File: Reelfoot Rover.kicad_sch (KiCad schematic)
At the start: 2 parts, among them J1 GPIO, U1 7432

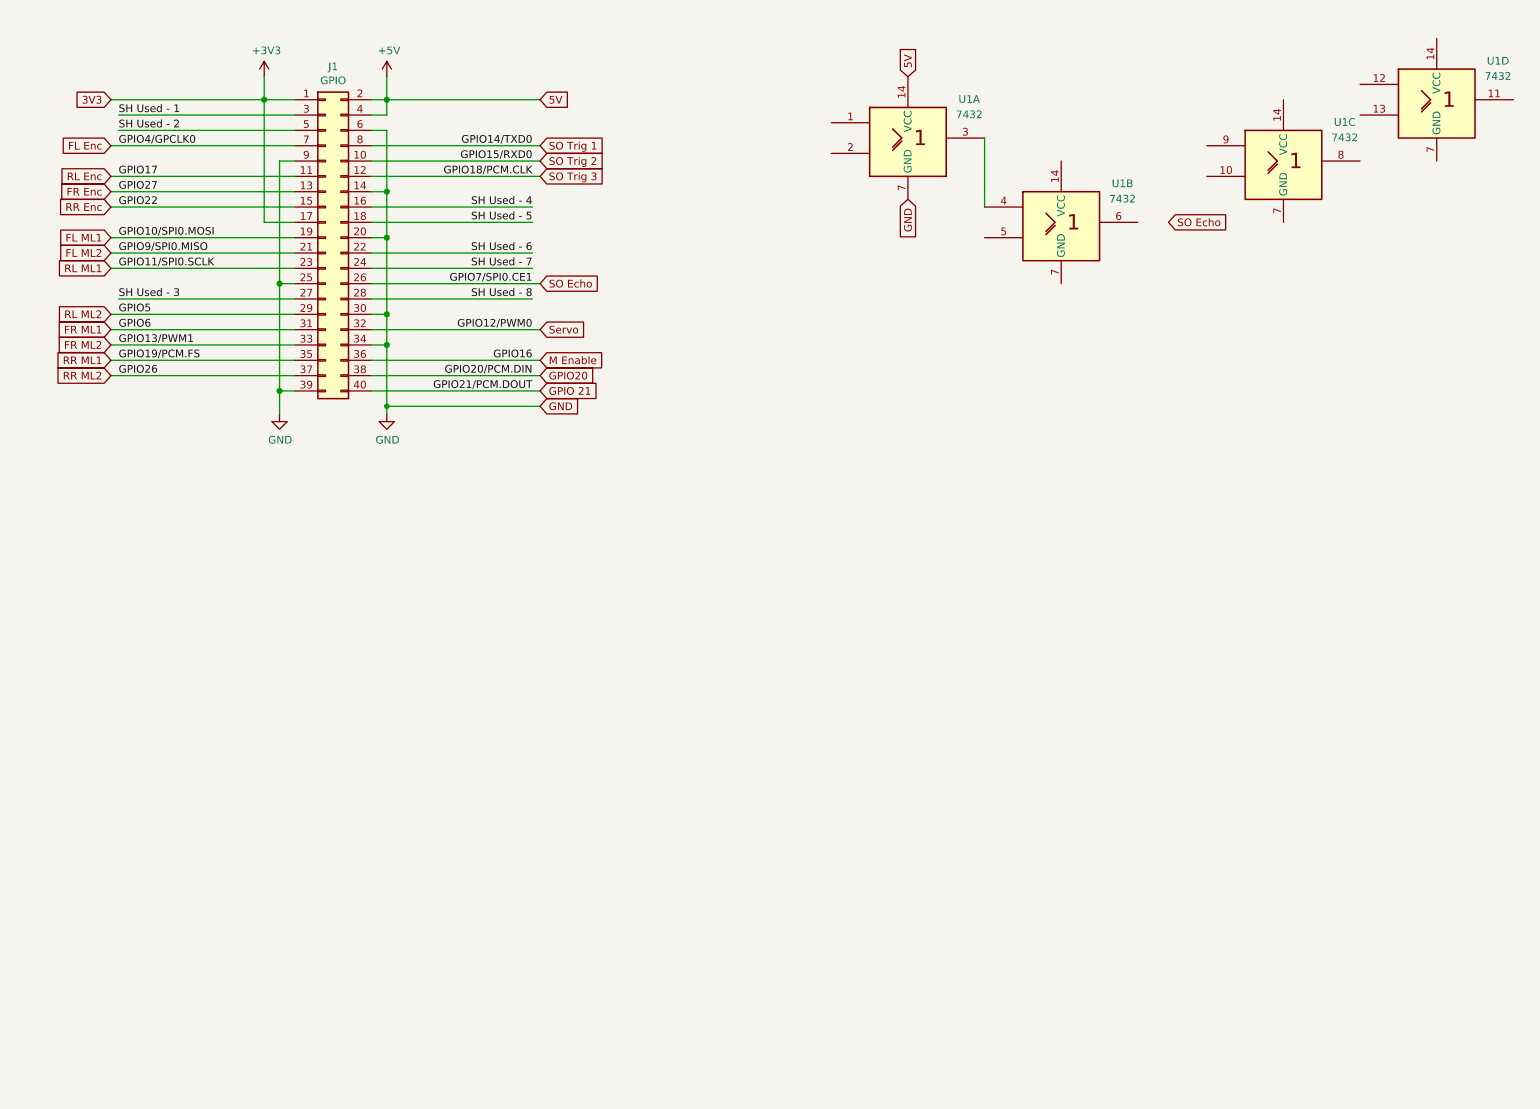
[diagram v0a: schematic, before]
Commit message: first complete draft
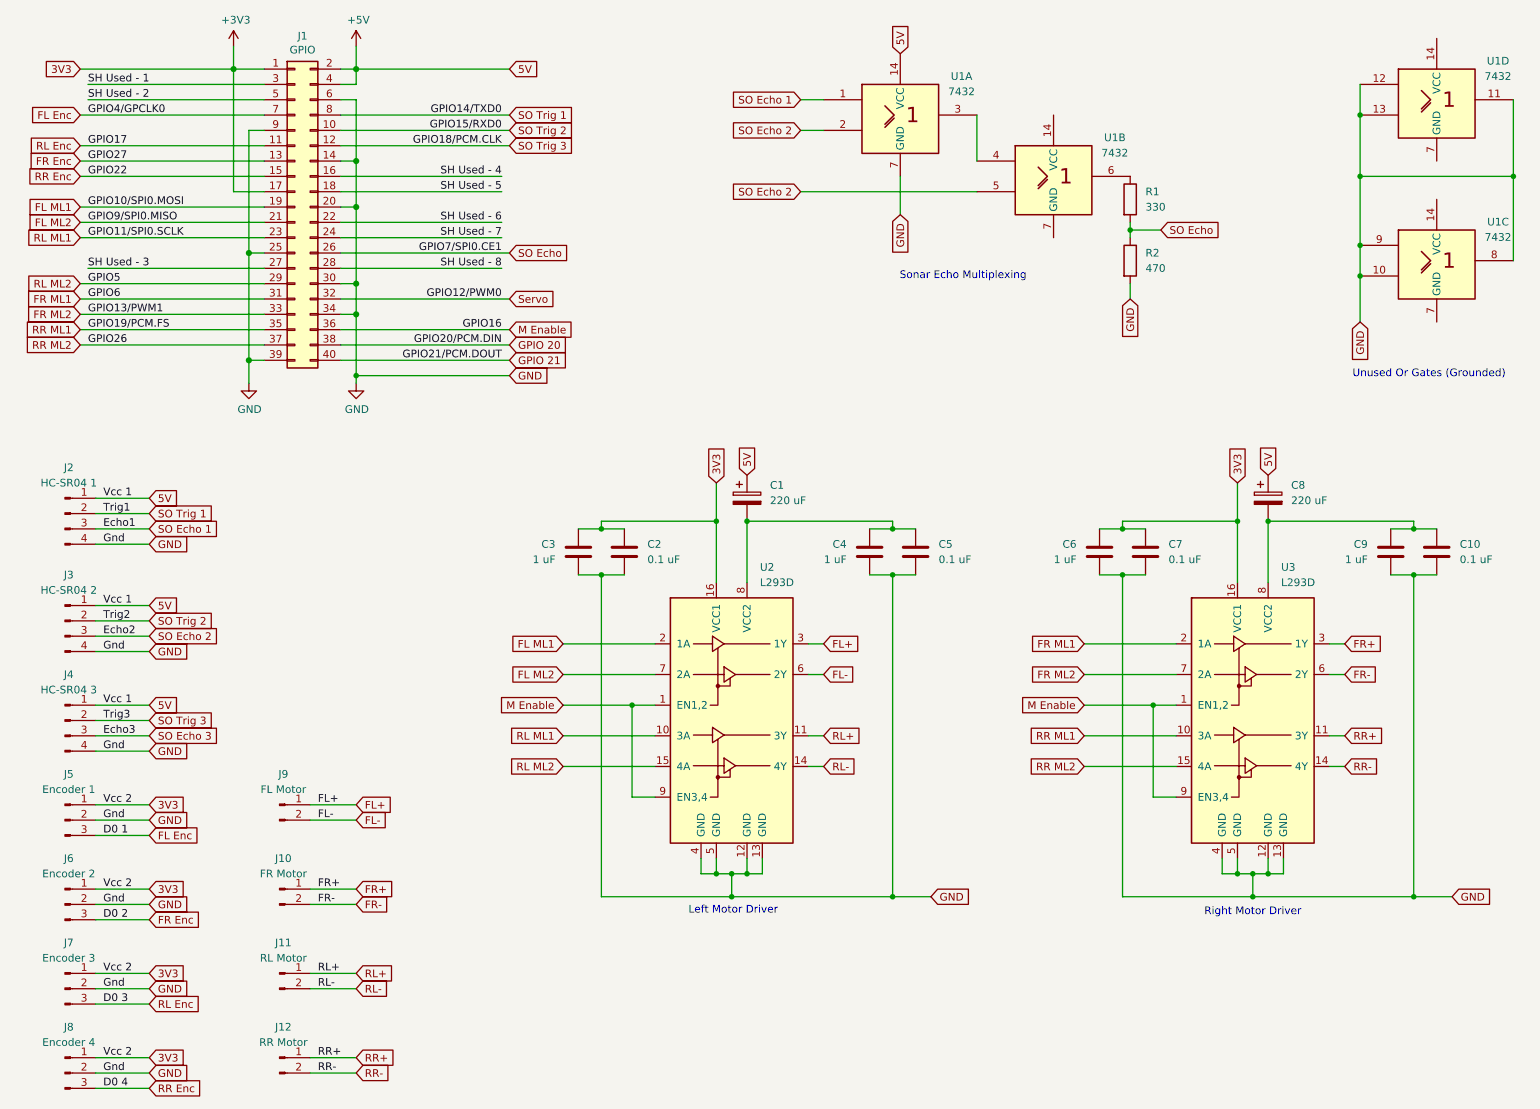
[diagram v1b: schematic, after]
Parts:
- added C1, C8: 220 uF, symbol Device:C_Polarized
- added C10, C2, C5, C7: 0.1 uF, symbol Device:C
- added C3, C4, C6, C9: 1 uF, symbol Device:C
- added J10: FR Motor, symbol Connector:Conn_01x02_Pin
- added J11: RL Motor, symbol Connector:Conn_01x02_Pin
- added J12: RR Motor, symbol Connector:Conn_01x02_Pin
- added J2: HC-SR04 1, symbol Connector:Conn_01x04_Pin
- added J3: HC-SR04 2, symbol Connector:Conn_01x04_Pin
- added J4: HC-SR04 3, symbol Connector:Conn_01x04_Pin
- added J5: Encoder 1, symbol Connector:Conn_01x03_Pin
- added J6: Encoder 2, symbol Connector:Conn_01x03_Pin
- added J7: Encoder 3, symbol Connector:Conn_01x03_Pin
- added J8: Encoder 4, symbol Connector:Conn_01x03_Pin
- added J9: FL Motor, symbol Connector:Conn_01x02_Pin
- added R1: 330, symbol Device:R
- added R2: 470, symbol Device:R
- added U2, U3: L293D, Package_DIP:DIP-16_W7.62mm, symbol Driver_Motor:L293D
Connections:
- net +3V3: now also C2.1, C3.1, C6.1, C7.1, J5.1 (Pin_1), J6.1 (Pin_1), J7.1 (Pin_1), J8.1 (Pin_1), U2.16 (VCC1), U3.16 (VCC1)
- net +5V: now also C1.1, C8.1, J2.1 (Pin_1), J3.1 (Pin_1), J4.1 (Pin_1)
- net FL Enc: now also J5.3 (Pin_3)
- net FL ML1: now also U2.2 (1A)
- net FL ML2: now also U2.7 (2A)
- net FR Enc: now also J6.3 (Pin_3)
- net FR ML1: now also U3.2 (1A)
- net FR ML2: now also U3.7 (2A)
- net GND: now also U1.10, U1.11, U1.12, U1.13, U1.8, U1.9, C10.2, C2.2, C3.2, C4.2, C5.2, C6.2, C7.2, C9.2, J2.4 (Pin_4), J3.4 (Pin_4), J4.4 (Pin_4), J5.2 (Pin_2), J6.2 (Pin_2), J7.2 (Pin_2), J8.2 (Pin_2), R2.2, U2.12 (GND), U2.13 (GND), U2.4 (GND), U2.5 (GND), U3.12 (GND), U3.13 (GND), U3.4 (GND), U3.5 (GND)
- net M Enable: now also U2.1 (EN1,2), U2.9 (EN3,4), U3.1 (EN1,2), U3.9 (EN3,4)
- net RL Enc: now also J7.3 (Pin_3)
- net RL ML1: now also U2.10 (3A)
- net RL ML2: now also U2.15 (4A)
- net RR Enc: now also J8.3 (Pin_3)
- net RR ML1: now also U3.10 (3A)
- net RR ML2: now also U3.15 (4A)
- net SO Echo: now also R1.2, R2.1
- net SO Trig 1: now also J2.2 (Pin_2)
- net SO Trig 2: now also J3.2 (Pin_2)
- net SO Trig 3: now also J4.2 (Pin_2)
- net SO Echo 1: now reaches U1.1
- net SO Echo 1: now also J2.3 (Pin_3)
- net SO Echo 2: now reaches U1.2
- net SO Echo 2: now also U1.5, J3.3 (Pin_3)
- net at U1.6: now also R1.1
- net GPIO20 renamed GPIO 20
- new net: C1.2, C4.1, C5.1, U2.8 (VCC2)
- new net: C10.1, C8.2, C9.1, U3.8 (VCC2)
- new net FL+: J9.1 (Pin_1), U2.3 (1Y)
- new net FL-: J9.2 (Pin_2), U2.6 (2Y)
- new net FR+: J10.1 (Pin_1), U3.3 (1Y)
- new net FR-: J10.2 (Pin_2), U3.6 (2Y)
- new net RL+: J11.1 (Pin_1), U2.11 (3Y)
- new net RL-: J11.2 (Pin_2), U2.14 (4Y)
- new net RR+: J12.1 (Pin_1), U3.11 (3Y)
- new net RR-: J12.2 (Pin_2), U3.14 (4Y)
- new net SO Echo 3: J4.3 (Pin_3)
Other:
- note added: "Left Motor Driver"
- note added: "Right Motor Driver"
- note added: "Sonar Echo Multiplexing"
- note added: "Unused Or Gates (Grounded)"
- moved on the sheet: J1, U1A, U1B, U1C
